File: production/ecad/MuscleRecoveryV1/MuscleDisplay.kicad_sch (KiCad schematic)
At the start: 2 parts, among them J5 Conn_01x11_Pin, U8 ESP32-WROOM-32

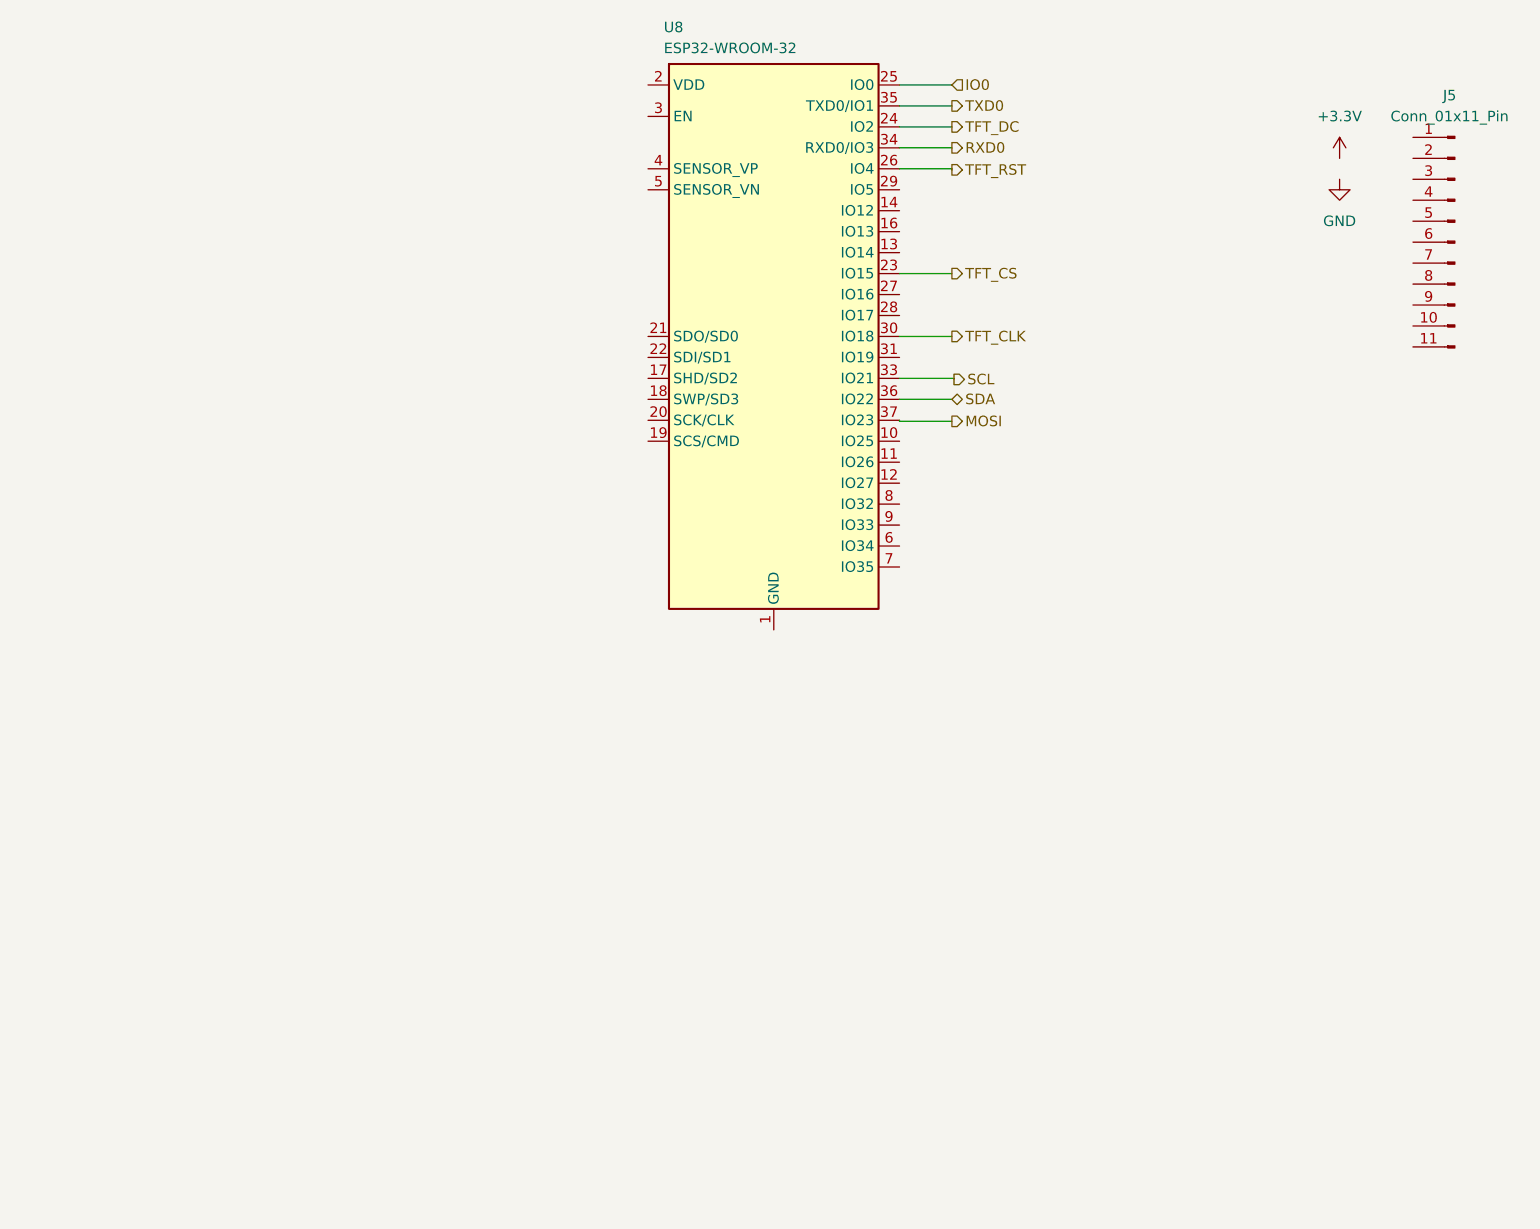
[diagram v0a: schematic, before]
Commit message: Revert "Display commit 1"
This reverts commit 52e50f7827ccbfa861bea7a8a003d131d02fed89.
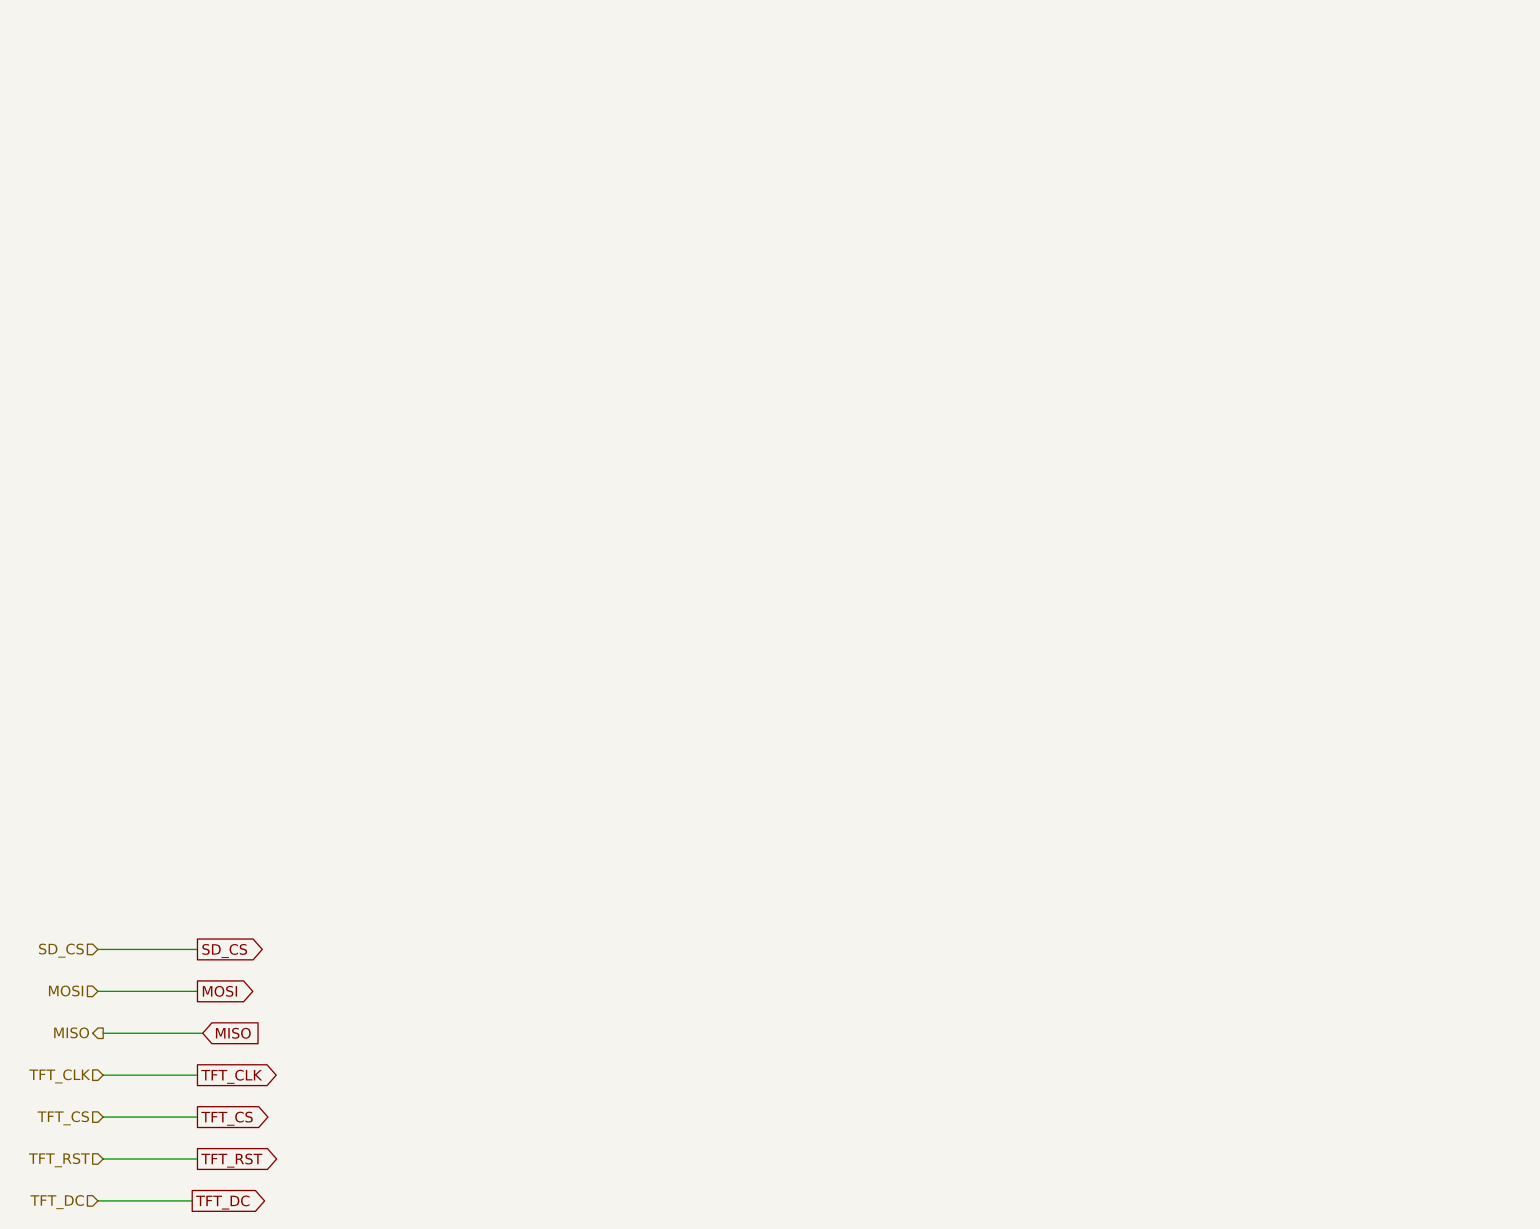
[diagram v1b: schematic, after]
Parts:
- removed J5: Conn_01x11_Pin, symbol Connector:Conn_01x11_Pin
- removed U8: ESP32-WROOM-32, RF_Module:ESP32-WROOM-32, symbol RF_Module:ESP32-WROOM-32

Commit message: Display commit 1
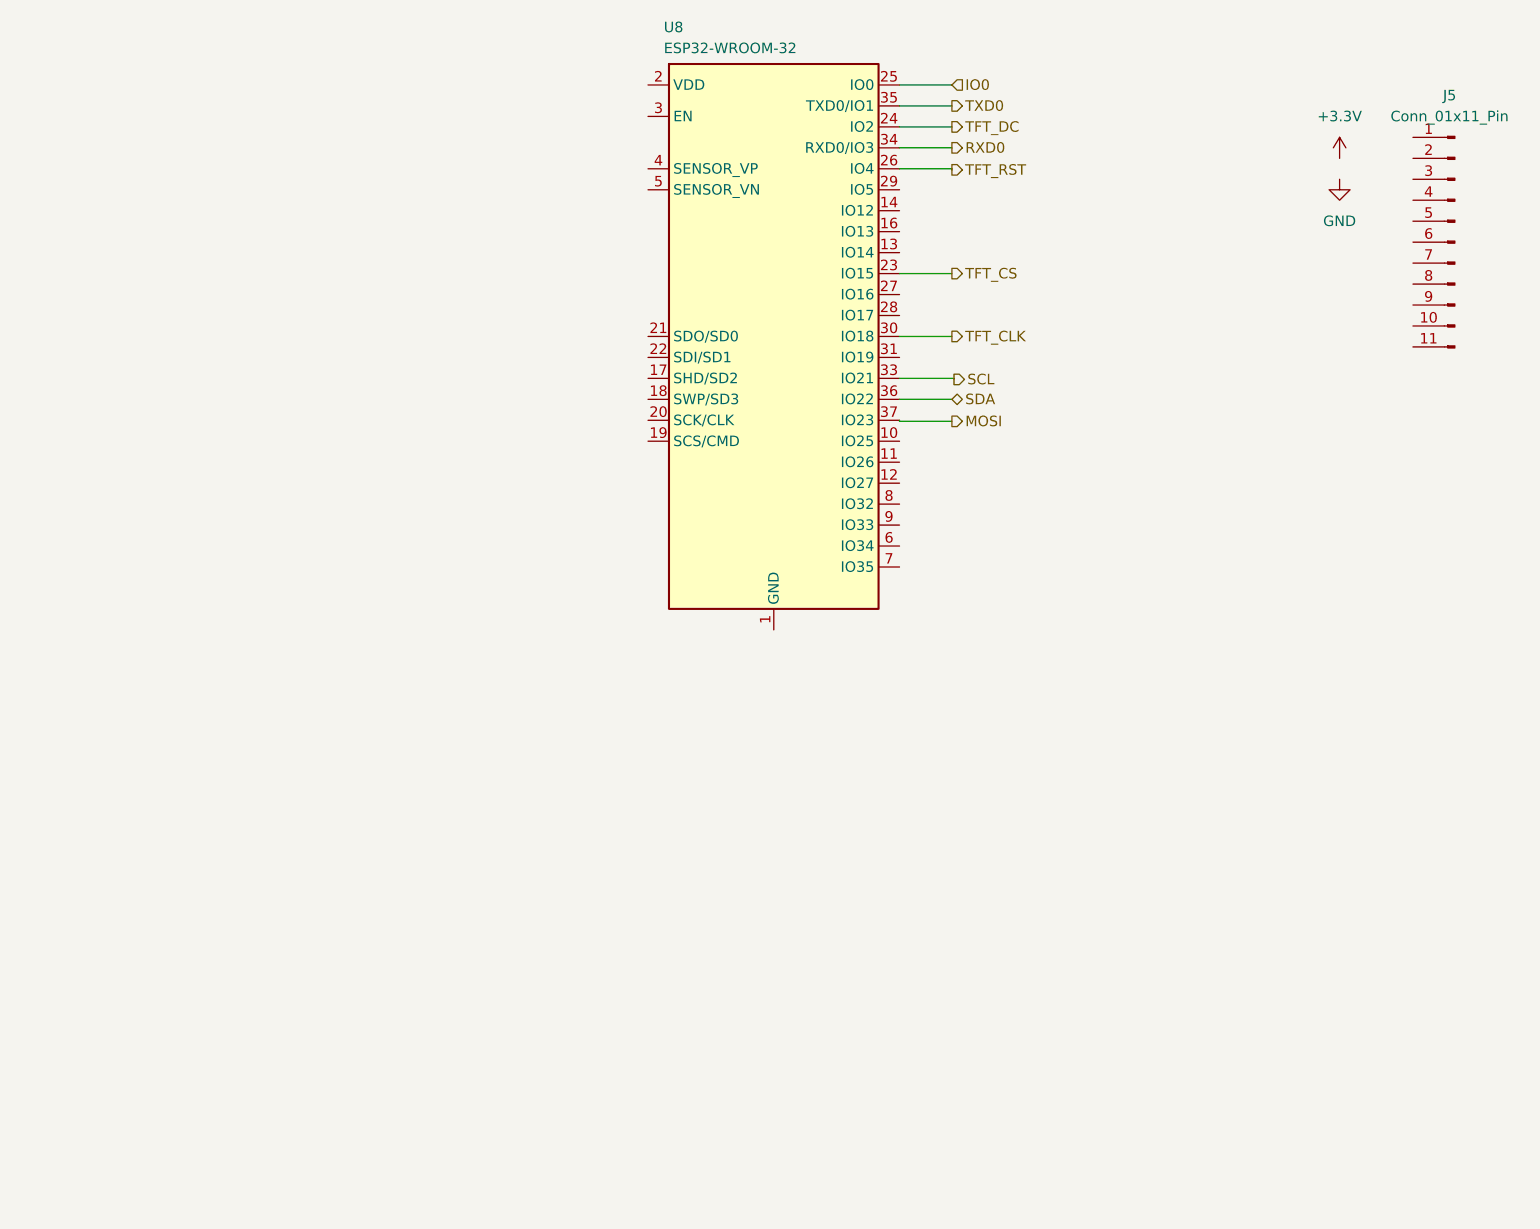
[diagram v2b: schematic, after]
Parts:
- added J5: Conn_01x11_Pin, symbol Connector:Conn_01x11_Pin
- added U8: ESP32-WROOM-32, RF_Module:ESP32-WROOM-32, symbol RF_Module:ESP32-WROOM-32
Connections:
- net MOSI: now also U8.37 (IO23)
- net TFT_CLK: now also U8.30 (IO18)
- net TFT_CS: now also U8.23 (IO15)
- net TFT_DC: now also U8.24 (IO2)
- net TFT_RST: now also U8.26 (IO4)
- new net: U8.1 (GND), U8.15 (GND), U8.38 (GND), U8.39 (GND)
- new net IO0: U8.25 (IO0)
- new net RXD0: U8.34 (RXD0/IO3)
- new net SCL: U8.33 (IO21)
- new net SDA: U8.36 (IO22)
- new net TXD0: U8.35 (TXD0/IO1)
